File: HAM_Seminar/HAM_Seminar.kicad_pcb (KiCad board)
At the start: 2 copper layers, 124 x 44 mm, 17 parts, among them J2 Conn_01x02_Socket, U1 NE555P, U2 74LS90, U3 74LS48, U4 MAN3840A

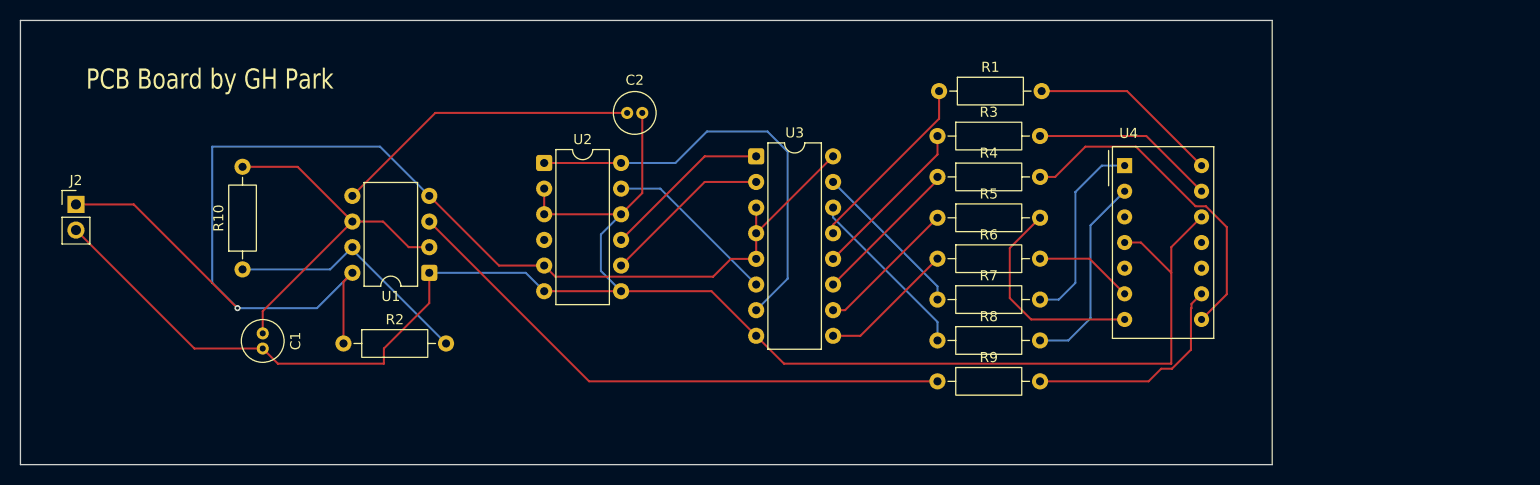
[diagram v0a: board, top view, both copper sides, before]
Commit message: sERT
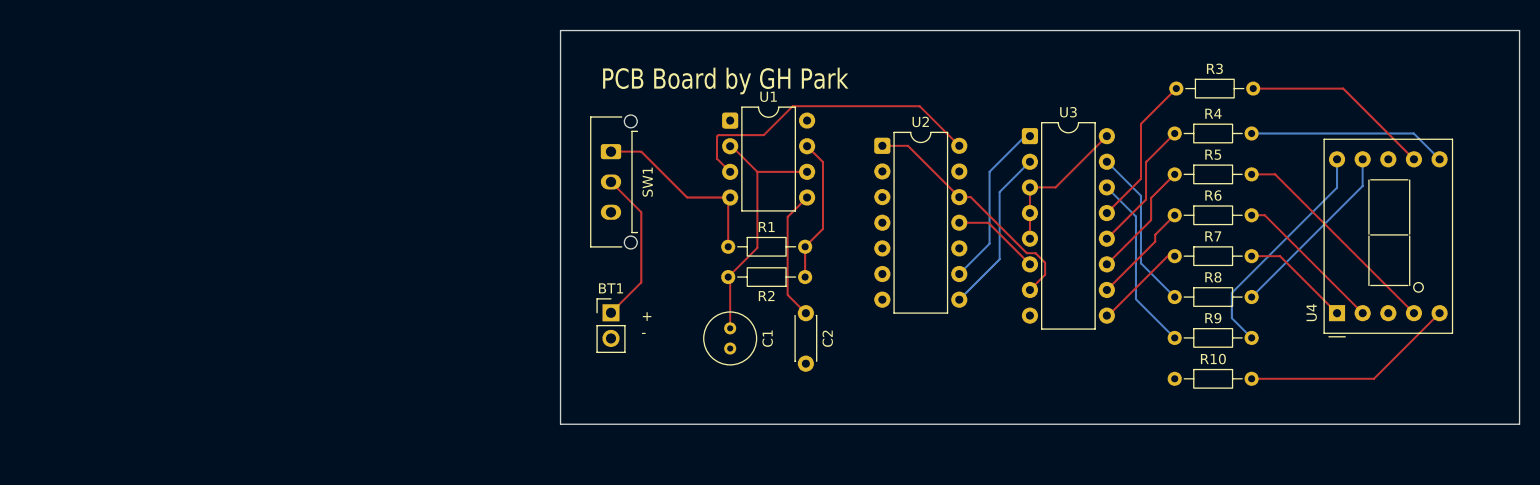
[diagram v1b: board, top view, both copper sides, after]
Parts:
- removed J2: Conn_01x02_Socket, Connector_PinHeader_2.54mm:PinHeader_1x02_P2.54mm_Vertical
- added BT1: Battery, Connector_PinHeader_2.54mm:PinHeader_1x02_P2.54mm_Vertical, F.Cu at (170.0, 101.0)
- added SW1: SW_SPDT, Connector_Molex:Molex_Micro-Fit_3.0_43650-0315_1x03_P3.00mm_Vertical, F.Cu at (170.0, 85.0)
- C1: footprint Capacitor_THT:C_Radial_D4.0mm_H7.0mm_P1.50mm -> Capacitor_THT:C_Radial_D5.0mm_H5.0mm_P2.00mm
- C2: footprint Capacitor_THT:C_Radial_D4.0mm_H7.0mm_P1.50mm -> Capacitor_THT:C_Disc_D4.3mm_W1.9mm_P5.00mm
- R1: renamed from R2; footprint Resistor_THT:R_Axial_DIN0207_L6.3mm_D2.5mm_P10.16mm_Horizontal -> Resistor_THT:R_Axial_DIN0204_L3.6mm_D1.6mm_P7.62mm_Horizontal
- R10: renamed from R9; footprint Resistor_THT:R_Axial_DIN0207_L6.3mm_D2.5mm_P10.16mm_Horizontal -> Resistor_THT:R_Axial_DIN0204_L3.6mm_D1.6mm_P7.62mm_Horizontal
- R2: renamed from R10; footprint Resistor_THT:R_Axial_DIN0207_L6.3mm_D2.5mm_P10.16mm_Horizontal -> Resistor_THT:R_Axial_DIN0204_L3.6mm_D1.6mm_P7.62mm_Horizontal
- R3: renamed from R1; footprint Resistor_THT:R_Axial_DIN0207_L6.3mm_D2.5mm_P10.16mm_Horizontal -> Resistor_THT:R_Axial_DIN0204_L3.6mm_D1.6mm_P7.62mm_Horizontal
- R4: renamed from R3; footprint Resistor_THT:R_Axial_DIN0207_L6.3mm_D2.5mm_P10.16mm_Horizontal -> Resistor_THT:R_Axial_DIN0204_L3.6mm_D1.6mm_P7.62mm_Horizontal
- R5: renamed from R4; footprint Resistor_THT:R_Axial_DIN0207_L6.3mm_D2.5mm_P10.16mm_Horizontal -> Resistor_THT:R_Axial_DIN0204_L3.6mm_D1.6mm_P7.62mm_Horizontal
- R6: renamed from R5; footprint Resistor_THT:R_Axial_DIN0207_L6.3mm_D2.5mm_P10.16mm_Horizontal -> Resistor_THT:R_Axial_DIN0204_L3.6mm_D1.6mm_P7.62mm_Horizontal
- R7: renamed from R6; footprint Resistor_THT:R_Axial_DIN0207_L6.3mm_D2.5mm_P10.16mm_Horizontal -> Resistor_THT:R_Axial_DIN0204_L3.6mm_D1.6mm_P7.62mm_Horizontal
- R8: renamed from R7; footprint Resistor_THT:R_Axial_DIN0207_L6.3mm_D2.5mm_P10.16mm_Horizontal -> Resistor_THT:R_Axial_DIN0204_L3.6mm_D1.6mm_P7.62mm_Horizontal
- R9: renamed from R8; footprint Resistor_THT:R_Axial_DIN0207_L6.3mm_D2.5mm_P10.16mm_Horizontal -> Resistor_THT:R_Axial_DIN0204_L3.6mm_D1.6mm_P7.62mm_Horizontal
- U2: footprint Package_DIP:DIP-12_W7.62mm -> Package_DIP:DIP-14_W7.62mm
- U4: value MAN3840A -> D148K; footprint Display_7Segment:MAN3810A -> Display_7Segment:D1X8K
- moved R2 55.7 mm to (189.2, 97.4), turned to 180 degrees
- moved C1 46.3 mm to (181.8, 102.5)
- moved R1 39.3 mm to (181.6, 94.4)
- moved U2 33.5 mm to (196.9, 84.4)
- moved U1 33.4 mm to (181.8, 81.9), turned to 0 degrees
- moved U3 27.2 mm to (211.5, 83.5)
- moved C2 26.6 mm to (189.3, 101.0), turned to -90 degrees
- moved U4 25.6 mm to (241.9, 101.0), turned to 90 degrees
- moved R10 23.5 mm to (225.8, 107.5)
- moved R3 23.5 mm to (226.0, 78.8)
- moved R4 23.5 mm to (225.8, 83.2)
- moved R5 23.5 mm to (225.8, 87.2)
- moved R6 23.5 mm to (225.8, 91.3)
- moved R7 23.5 mm to (225.8, 95.3)
- moved R8 23.5 mm to (225.8, 99.4)
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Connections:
- R10 pad 2: Net-(U4-D.P.) -> Net-(U4-DP)
- U4 pad 1: Net-(U4-F) -> Net-(U4-E)
- U4 pad 10: unconnected-(U4-NC-Pad10) -> Net-(U4-G)
- U4 pad 2: Net-(U4-G) -> Net-(U4-D)
- U4 pad 3: unconnected-(U4-NC-Pad3) -> GND
- U4 pad 4: GND -> Net-(U4-C)
- U4 pad 5: unconnected-(U4-NC-Pad5) -> Net-(U4-DP)
- U4 pad 6: Net-(U4-E) -> Net-(U4-B)
- U4 pad 7: Net-(U4-D) -> Net-(U4-A)
- U4 pad 8: Net-(U4-C) -> GND
- U4 pad 9: Net-(U4-D.P.) -> Net-(U4-F)
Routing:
- net GND: track 176.1 -> 0.00 mm
- net VCC: track 133.3 -> 33.5 mm, vias 1 -> 0
- net Net-(U1-Q): track 56.9 -> 30.9 mm
- net Net-(U4-D.P.): track 22.2 -> 0.00 mm
- net Net-(U4-DP): track 0.00 -> 21.3 mm
- net Net-(U2-CP1..3): track 43.2 -> 24.2 mm
- net Net-(U1-CV): track 30.6 -> 13.0 mm
- net Net-(BT1-+): track 0.00 -> 15.4 mm
- net Net-(U4-C): track 33.2 -> 21.8 mm
- net Net-(U1-THR): track 36.6 -> 25.4 mm
- net Net-(U1-DIS): track 25.2 -> 14.3 mm
- net Net-(U2-Q3): track 17.3 -> 8.71 mm
- net Net-(U4-D): track 21.5 -> 15.0 mm
- net Net-(U3-e): track 13.5 -> 9.16 mm
- net Net-(U3-d): track 14.1 -> 10.2 mm
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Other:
- board size 124 x 44 mm -> 95 x 39 mm
- board text added: "+ -"
- board text removed: "${REFERENCE}"
